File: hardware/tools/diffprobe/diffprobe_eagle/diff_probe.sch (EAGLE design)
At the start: 24 parts, among them U1 AD8129, X1 SMA-142-0701-801/806

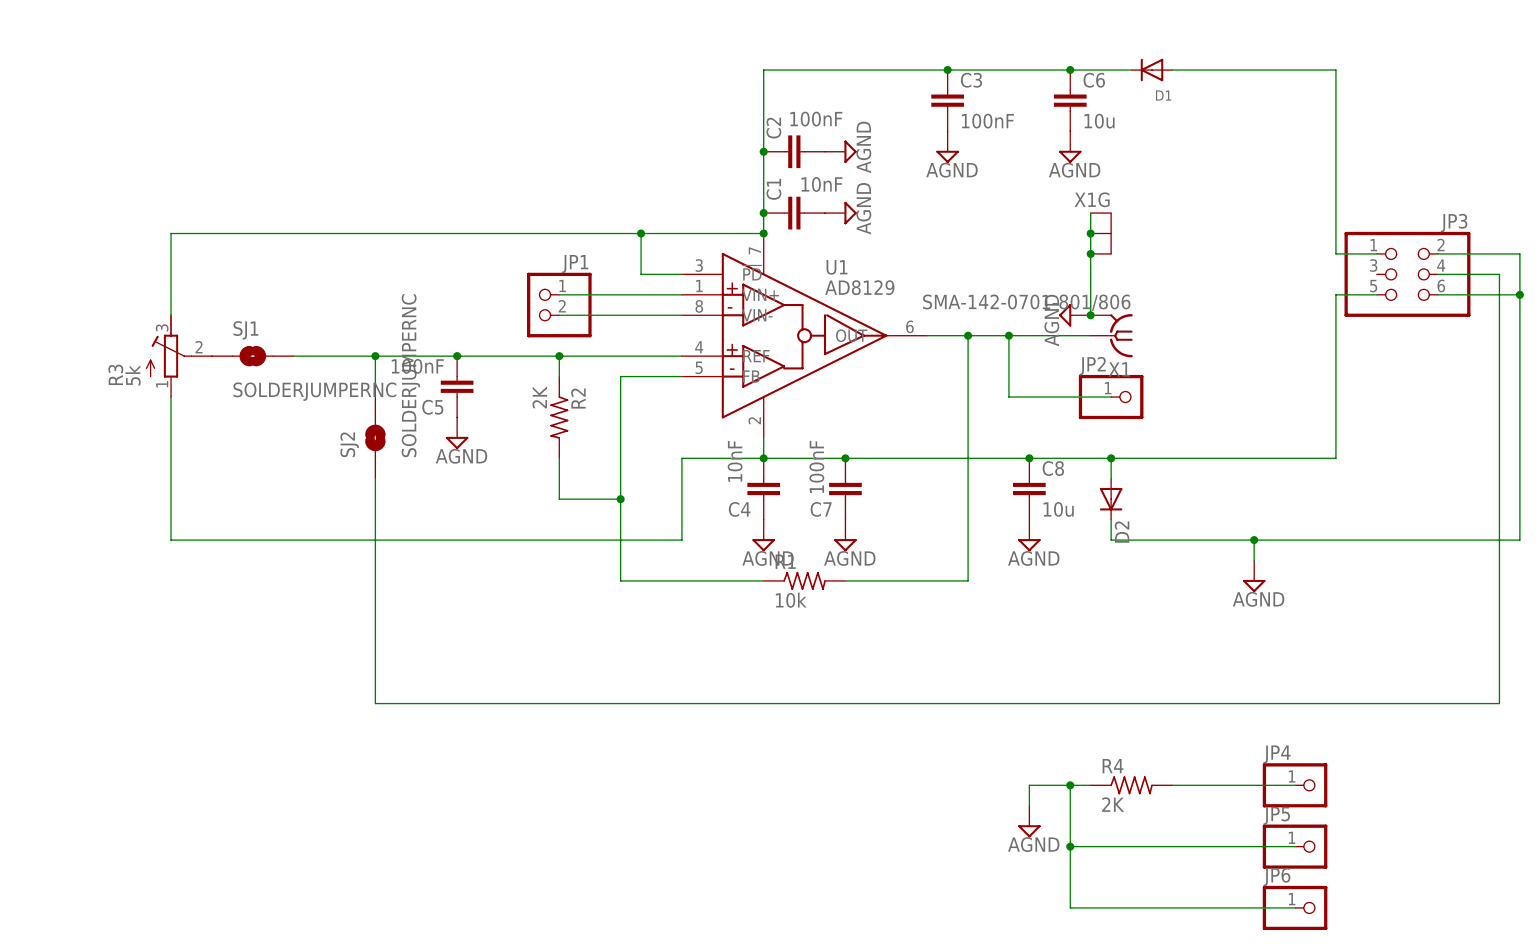
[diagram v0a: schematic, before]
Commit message: Fix issues with differential probe
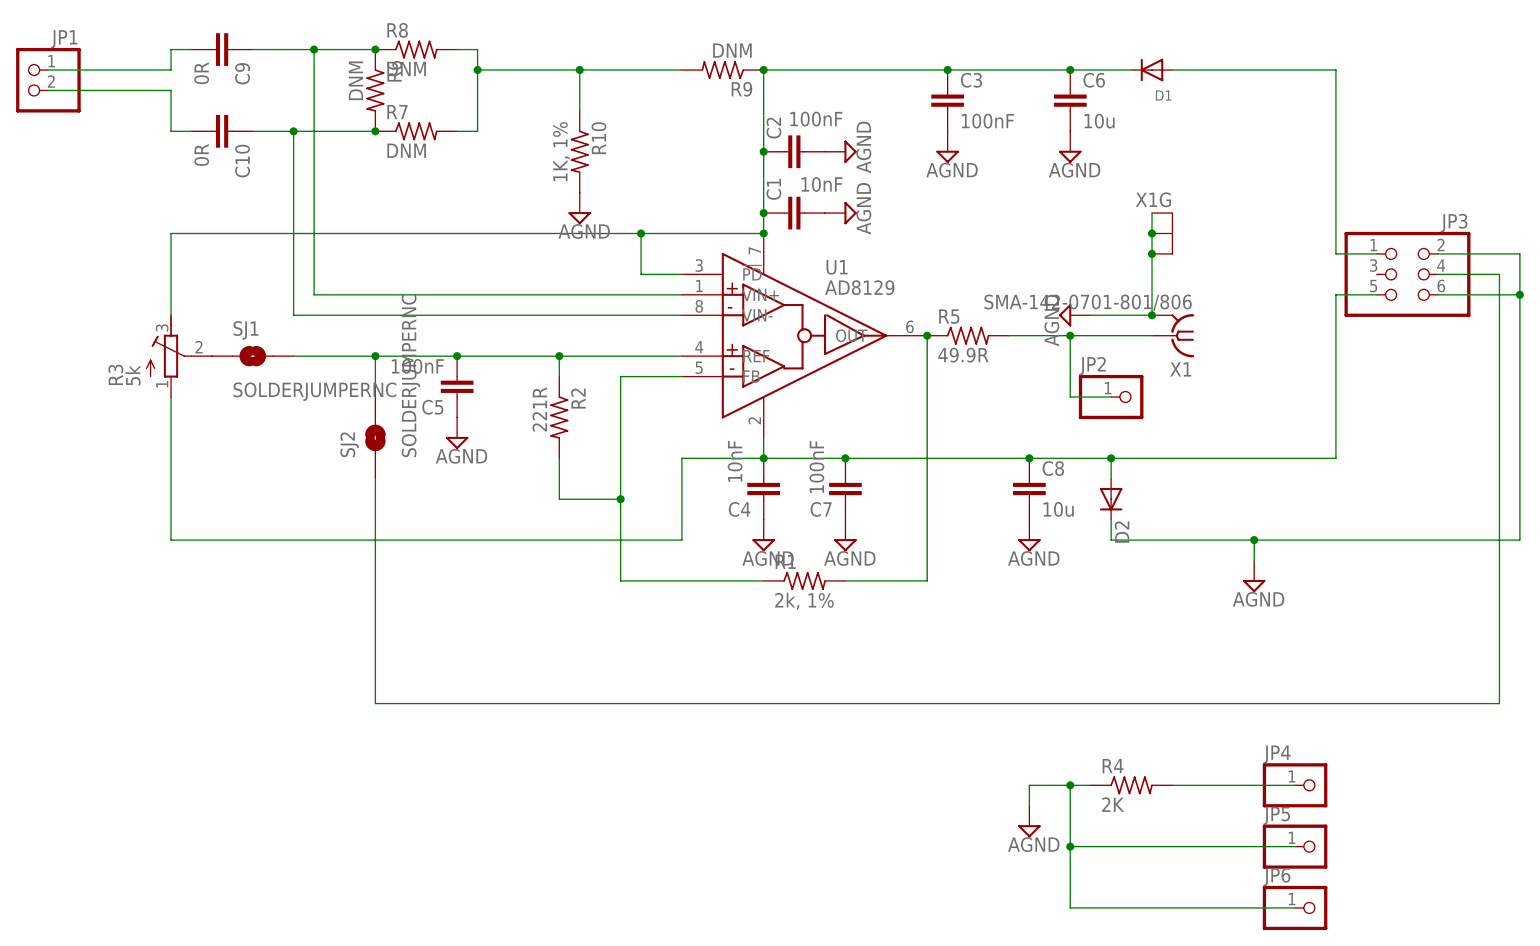
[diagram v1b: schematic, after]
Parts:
- added C10, C9: 0R, rcl:C-EUC0603
- added R10: 1K, 1%, resistor:R-US_R0603
- added R5: 49.9R, resistor:R-US_R0603
- added R6: DNM, resistor:R-US_M0805
- added R7, R8, R9: DNM, resistor:R-US_R0603
- R1: value 10k -> 2k, 1%
- R2: value 2K -> 221R
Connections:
- new net N$12: JP2.1, R5.2, X1G1.1
- new net N$13: C10.1, R6.2, R7.1, U1.VIN-
- new net N$14: C10.2, JP1.2
- new net N$15: R10.1, R7.2, R8.2, R9.2
- net AGND: now also R10.2
- net N$2: now also R9.1
- net N$5: now also R5.1; no longer JP2.1, X1G1.1
- net N$6: now also C9.2; no longer U1.VIN+
- net N$7: now also C9.1, R6.1, R8.1, U1.VIN+; no longer JP1.2, U1.VIN-
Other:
- moved on the sheet: JP1, X1, X1G
